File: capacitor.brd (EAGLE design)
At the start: 15.3 x 29.3 mm, 3 parts

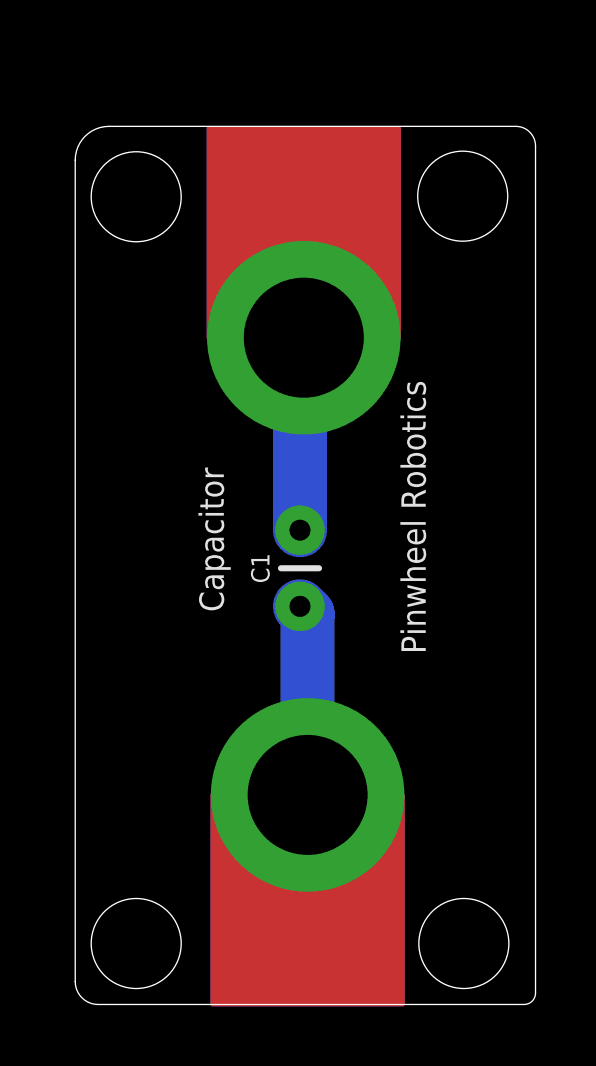
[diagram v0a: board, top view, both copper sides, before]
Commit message: New Updates
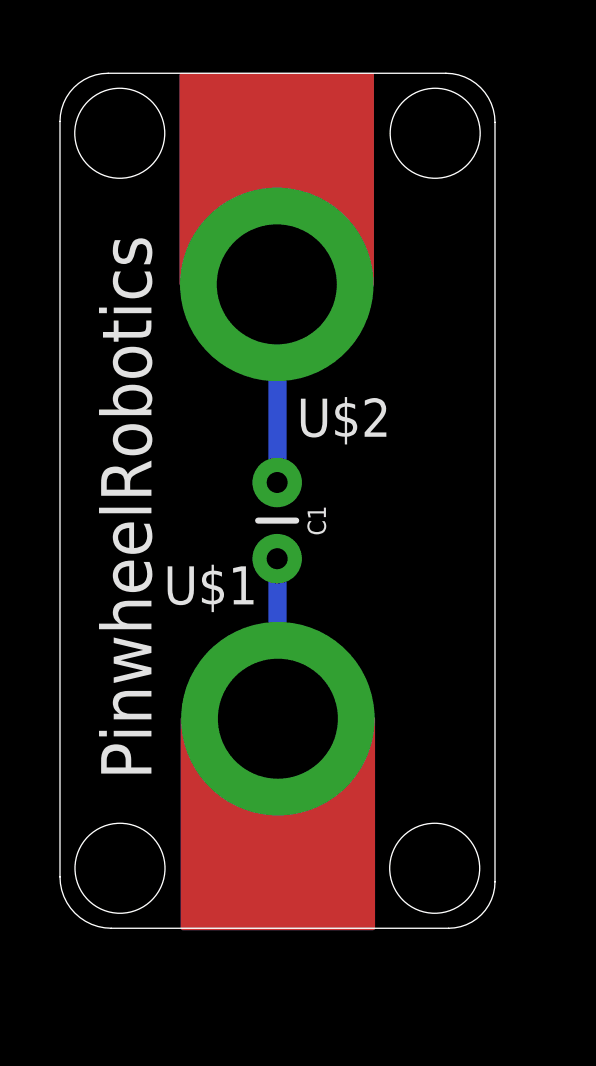
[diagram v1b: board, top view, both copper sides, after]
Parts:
- moved U$2 17.0 mm to (7.23, 21.5), turned to 180 degrees
- moved U$1 12.7 mm to (7.26, 6.99), turned to 0 degrees
- moved C1 1.76 mm to (7.24, 13.6), turned to 270 degrees
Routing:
- net N$2: track 6.27 -> 5.34 mm
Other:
- board size 15.3 x 29.3 mm -> 14.5 x 28.5 mm
- board text added: "PinwheelRobotics"
- board text added: "care@pinwheel.in"
- board text removed: "Capacitor"
- board text removed: "Pinwheel Robotics"
- board text removed: "care@Pinwheel.in"
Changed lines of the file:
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@@
 <board>
 <plain>
-<wire x1="0.508" y1="25.60563125" x2="0.508" y2="-1.778" width="0" layer="20"/>
-<wire x1="0.508" y1="-1.778" x2="1.27" y2="-2.54" width="0" layer="20" curve="90"/>
-<wire x1="1.27" y1="-2.54" x2="15.47" y2="-2.54" width="0" layer="20"/>
-<wire x1="15.47" y1="-2.54" x2="15.851" y2="-2.159" width="0" layer="20" curve="90"/>
-<wire x1="15.851" y1="-2.159" x2="15.851" y2="26.075184375" width="0" layer="20"/>
-<wire x1="15.851" y1="26.075184375" x2="15.196184375" y2="26.73" width="0" layer="20" curve="90"/>
-<wire x1="15.196184375" y1="26.73" x2="1.63236875" y2="26.73" width="0" layer="20"/>
-<wire x1="1.63236875" y1="26.73" x2="0.508" y2="25.60563125" width="0" layer="20" curve="90"/>
-<text x="12.192" y="9.144" size="0.8128" layer="21" rot="R90">Pinwheel Robotics </text>
-<text x="5.461" y="10.541" size="0.8128" layer="21" rot="R90">Capacitor</text>
-<text x="5.08" y="20.32" size="1.778" layer="22" rot="MR270">care@Pinwheel.in</text>
-<hole x="13.462" y="-0.508" drill="3"/>
-<hole x="2.54" y="-0.508" drill="3"/>
-<hole x="13.424" y="24.403" drill="3"/>
-<hole x="2.54" y="24.384" drill="3"/>
-<dimension x1="1.040003125" y1="-0.5102625" x2="4.039996875" y2="-0.5057375" x3="2.500015625" y3="26" textsize="1.778" layer="20" dtype="diameter"/>
-<dimension x1="2.54" y1="25.884" x2="2.54" y2="22.884" x3="15.113" y3="24.384" textsize="1.778" layer="20" dtype="diameter"/>
-<dimension x1="14.923996875" y1="24.40675" x2="11.924003125" y2="24.39925" x3="13.500003125" y3="-6" textsize="1.778" layer="20" dtype="diameter"/>
+<wire x1="14.5" y1="1.546503125" x2="14.5" y2="26.8651625" width="0" layer="20"/>
+<wire x1="14.5" y1="26.8651625" x2="12.8651625" y2="28.5" width="0" layer="20" curve="90"/>
+<wire x1="12.8651625" y1="28.5" x2="1.604278125" y2="28.5" width="0" layer="20"/>
+<wire x1="1.604278125" y1="28.5" x2="0" y2="26.895721875" width="0" layer="20" curve="90"/>
+<wire x1="0" y1="26.895721875" x2="0" y2="1.711603125" width="0" layer="20"/>
+<wire x1="0" y1="1.711603125" x2="1.711603125" y2="0" width="0" layer="20" curve="90"/>
+<wire x1="1.711603125" y1="0" x2="12.953496875" y2="0" width="0" layer="20"/>
+<wire x1="12.953496875" y1="0" x2="14.5" y2="1.546503125" width="0" layer="20" curve="90"/>
+<hole x="1.992" y="26.5" drill="3"/>
+<hole x="12.506" y="26.5" drill="3"/>
+<hole x="12.49" y="2" drill="3"/>
+<hole x="2" y="2" drill="3"/>
+<text x="3.048" y="4.953" size="1.6764" layer="21" rot="R90">PinwheelRobotics </text>
+<text x="13.716" y="23.368" size="1.6764" layer="22" rot="MR270">care@pinwheel.in</text>
 </plain>
 <attributes>
@@
 <autorouter>
 <pass name="Default">
-<param name="RoutingGrid" value="50mil"/>
+<param name="RoutingGrid" value="0.25mm"/>
 <param name="AutoGrid" value="1"/>
 <param name="Efforts" value="0"/>
@@
 </autorouter>
 <elements>
-<element name="C1" library="SparkFun-Capacitors" library_urn="urn:adsk.eagle:library:510" package="CAP-PTH-2.54" package3d_urn="urn:adsk.eagle:package:37435/1" value="22pF" x="8" y="12" smashed="yes" rot="R90">
-<attribute name="NAME" x="6.984" y="12" size="0.6096" layer="25" font="vector" ratio="20" rot="R90" align="bottom-center"/>
-<attribute name="PROD_ID" value="CAP-09128" x="25.78" y="27.24" size="1.778" layer="27" rot="R90" display="off"/>
-<attribute name="VALUE" x="9.016" y="12" size="0.6096" layer="27" font="vector" ratio="20" rot="R90" align="top-center"/>
+<element name="C1" library="SparkFun-Capacitors" library_urn="urn:adsk.eagle:library:510" package="CAP-PTH-2.54" package3d_urn="urn:adsk.eagle:package:37435/1" value="22pF" x="7.239" y="13.589" smashed="yes" rot="R270">
+<attribute name="NAME" x="8.255" y="13.589" size="0.6096" layer="25" font="vector" ratio="20" rot="R270" align="bottom-center"/>
+<attribute name="PROD_ID" value="CAP-09128" x="-10.541" y="-16.891" size="1.778" layer="27" rot="R270" display="off"/>
+<attribute name="VALUE" x="6.223" y="13.589" size="0.6096" layer="27" font="vector" ratio="20" rot="R270" align="top-center"/>
 </element>
-<element name="U$1" library="microbit" package="MICROBIT_PAD" value="MICROBIT_PAD" x="8.127" y="19.685" smashed="yes" rot="R180"/>
-<element name="U$2" library="microbit" package="MICROBIT_PAD" value="MICROBIT_PAD" x="8.254" y="4.445" smashed="yes"/>
+<element name="U$1" library="microbit" package="MICROBIT_PAD" value="MICROBIT_PAD" x="7.263" y="6.985" smashed="yes">
+<attribute name="NAME" x="3.453" y="10.795" size="1.27" layer="21"/>
+</element>
+<element name="U$2" library="microbit" package="MICROBIT_PAD" value="MICROBIT_PAD" x="7.2263" y="21.463" smashed="yes" rot="R180">
+<attribute name="NAME" x="11.0363" y="17.653" size="1.27" layer="21" rot="R180"/>
+</element>
 </elements>
 <signals>
@@
 <contactref element="C1" pad="1"/>
 <contactref element="U$2" pad="PAD"/>
-<wire x1="8.0772" y1="10.8204" x2="8" y2="10.73" width="0.1524" layer="16"/>
-<wire x1="8" y1="10.73" x2="8.254" y2="10.476" width="1.8" layer="16"/>
-<wire x1="8.254" y1="10.476" x2="8.254" y2="4.445" width="1.8" layer="16"/>
+<wire x1="7.25" y1="21.25" x2="7.25" y2="15" width="0.6096" layer="16"/>
+<wire x1="7.25" y1="15" x2="7.239" y2="14.859" width="0.1524" layer="16"/>
+<wire x1="7.25" y1="21.25" x2="7.2263" y2="21.463" width="0.1524" layer="16"/>
 </signal>
 <signal name="N$2">
 <contactref element="U$1" pad="PAD"/>
 <contactref element="C1" pad="2"/>
-<wire x1="8.0772" y1="13.5636" x2="8" y2="13.27" width="0.1524" layer="16"/>
-<wire x1="8.0772" y1="18.4404" x2="8.096790625" y2="18.459990625" width="0.1524" layer="16"/>
-<wire x1="8.096790625" y1="18.459990625" x2="8.127" y2="19.685" width="0" layer="19" extent="16-16"/>
-<wire x1="7.62" y1="19.05" x2="8.096790625" y2="18.459990625" width="0" layer="19" extent="16-16"/>
-<wire x1="8" y1="13.27" x2="8" y2="18.67" width="1.8" layer="16"/>
-<wire x1="8" y1="18.67" x2="7.62" y2="19.05" width="1.8" layer="16"/>
+<wire x1="7.25" y1="7" x2="7.25" y2="12.25" width="0.6096" layer="16"/>
+<wire x1="7.25" y1="12.25" x2="7.239" y2="12.319" width="0.1524" layer="16"/>
+<wire x1="7.25" y1="7" x2="7.263" y2="6.985" width="0.1524" layer="16"/>
 </signal>
 </signals>

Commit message: New Update
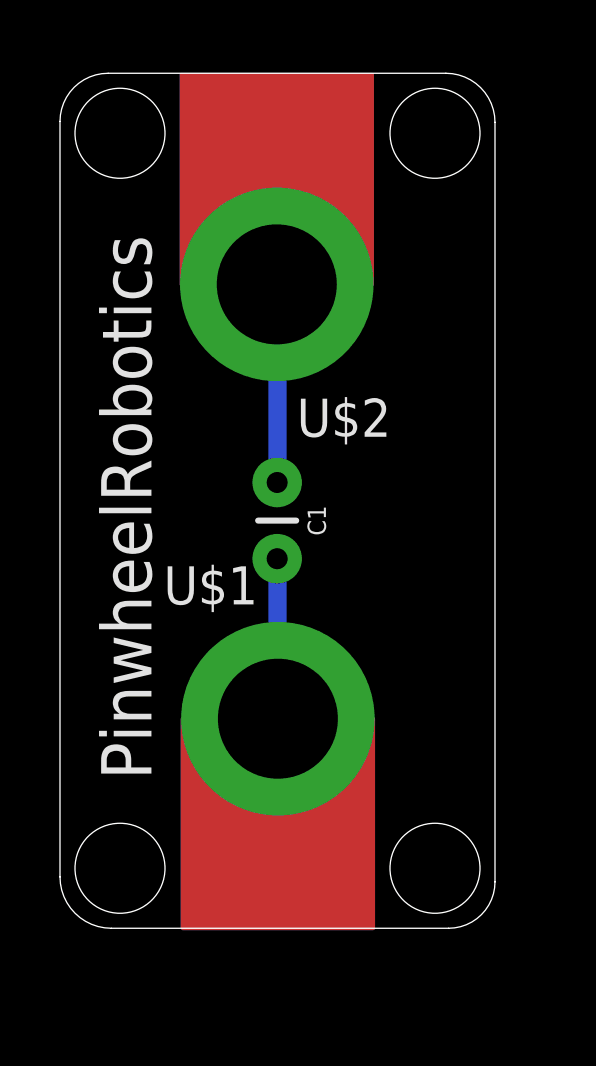
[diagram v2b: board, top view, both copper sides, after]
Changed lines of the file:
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@@
 <drawing>
 <settings>
-<setting alwaysvectorfont="yes"/>
+<setting alwaysvectorfont="no"/>
 <setting verticaltext="up"/>
 </settings>
@@
 <wire x1="1.711603125" y1="0" x2="12.953496875" y2="0" width="0" layer="20"/>
 <wire x1="12.953496875" y1="0" x2="14.5" y2="1.546503125" width="0" layer="20" curve="90"/>
-<hole x="1.992" y="26.5" drill="3"/>
-<hole x="12.506" y="26.5" drill="3"/>
-<hole x="12.49" y="2" drill="3"/>
+<hole x="2" y="26.5" drill="3"/>
+<hole x="12.5" y="26.5" drill="3"/>
+<hole x="12.5" y="2" drill="3"/>
 <hole x="2" y="2" drill="3"/>
 <text x="3.048" y="4.953" size="1.6764" layer="21" rot="R90">PinwheelRobotics </text>
